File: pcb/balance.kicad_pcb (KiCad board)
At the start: 2 copper layers, 7 x 6 mm, 42 parts, among them J1 Resistive_Touch, J2 JTAG, J3 Conn_01x04_Male, J4 PJ-102AH, J5 UART (Bluetooth), J6 Conn_02x03_Top_Bottom, J7 Conn_02x05_Top_Bottom, M1 Motor_Servo, M2 Motor_Servo, Q1 MMBT3904, Q2 MMBT3904, Q3 MMBT3904, SW1 SW_Push, U1 TM4C123GH6PMI, U2 LM2937xS, Y1 16MHz

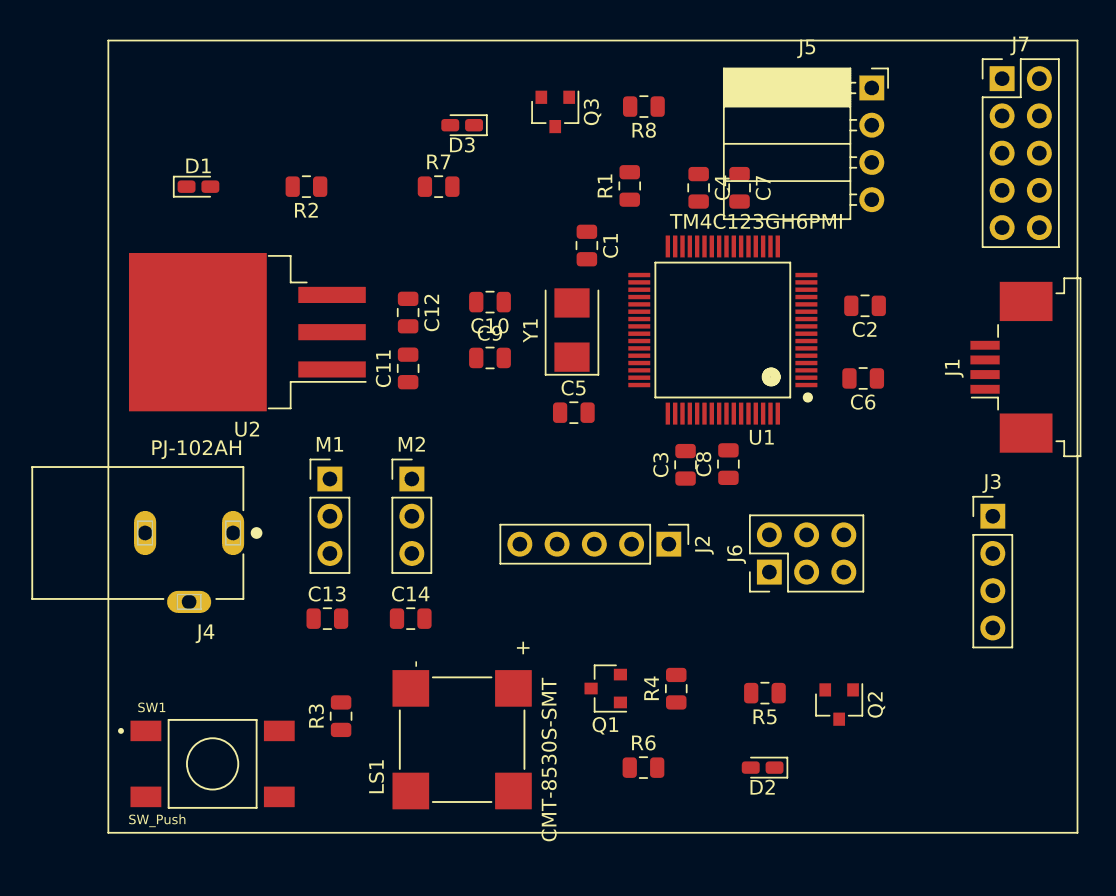
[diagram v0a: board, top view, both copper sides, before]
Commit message: Route the board
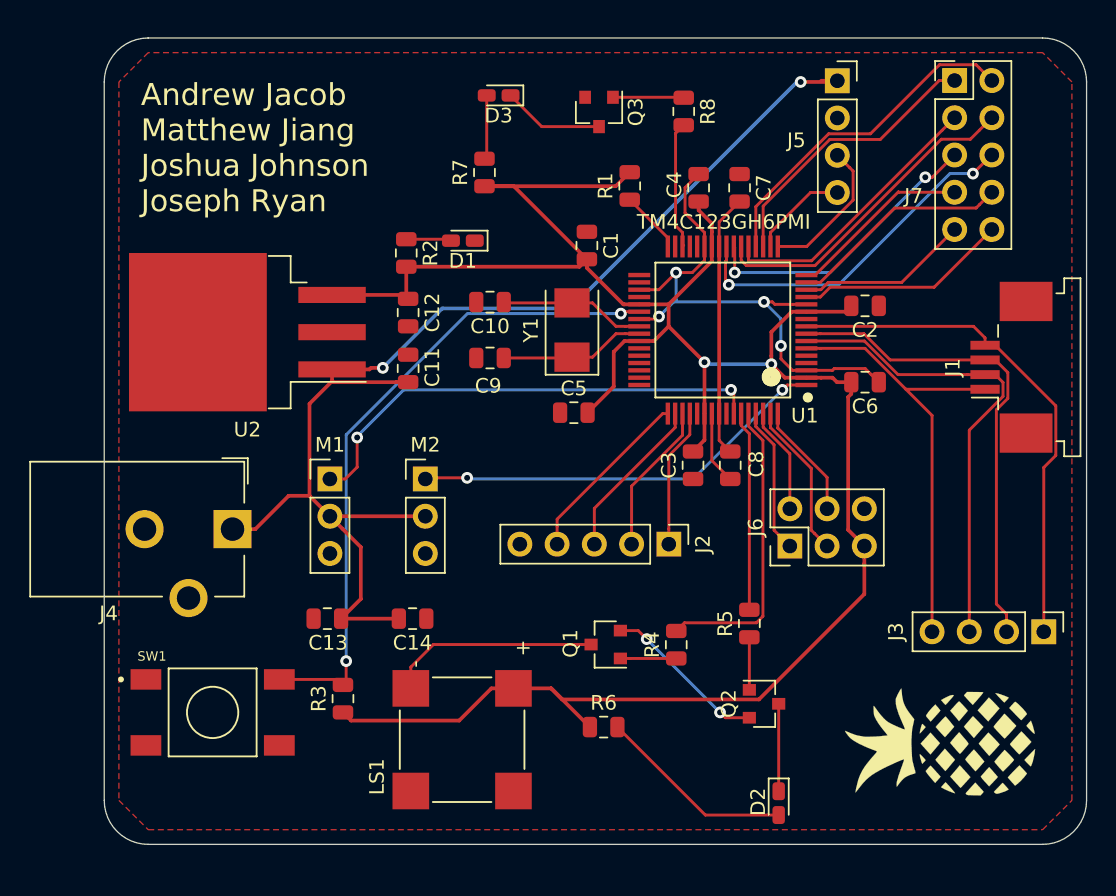
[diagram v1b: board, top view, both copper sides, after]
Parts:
- added G***: LOGO, pineapple:pineapple, F.Cu at (138.0, 150.0)
- J4: value PJ-102AH -> Barrel_Jack_Switch; footprint PJ-102AH:CUI_PJ-102AH -> Connector_BarrelJack:BarrelJack_CUI_PJ-102AH_Horizontal
- J5: footprint Connector_PinSocket_2.54mm:PinSocket_1x04_P2.54mm_Horizontal -> Connector_PinSocket_2.54mm:PinSocket_1x04_P2.54mm_Vertical
- moved D1 18.4 mm to (105.5, 115.8), turned to 180 degrees
- moved J3 8.61 mm to (145.1, 142.5), turned to 270 degrees
- moved R2 8.18 mm to (101.6, 116.7), turned to 90 degrees
- moved J4 6.47 mm to (89.8, 135.5), turned to 270 degrees
- moved Q2 5.13 mm to (126.0, 147.4), turned to 0 degrees
- moved R5 4.86 mm to (125.0, 141.9), turned to 90 degrees
- moved R6 3.88 mm to (115.1, 149.0)
- moved SW1 3.51 mm to (88.4, 148.0)
- moved R7 3.27 mm to (106.9, 111.2), turned to 90 degrees
- moved J7 3.24 mm to (139.0, 104.9)
- moved D3 3.21 mm to (107.9, 105.9)
- moved Q1 3.00 mm to (115.2, 143.4)
- moved R4 3.00 mm to (120.0, 143.4)
- moved Q3 2.99 mm to (114.7, 107.0)
- moved R8 2.74 mm to (120.5, 107.0), turned to 90 degrees
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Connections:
- J7 pad 8: /PC6 -> /PC5
- U1 pad 15: (no net) -> /PC5
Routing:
- net +3V3: track 0.00 -> 153.6 mm, vias 0 -> 2
- net +5V: track 0.00 -> 87.0 mm, vias 0 -> 2
- net GND: track 0.00 -> 54.2 mm, vias 0 -> 6
- net /RESET: track 0.00 -> 45.1 mm, vias 0 -> 2
- net Net-(J1-Pad4): track 0.00 -> 35.3 mm
- net Net-(J1-Pad3): track 0.00 -> 33.1 mm
- net /Servo0: track 0.00 -> 32.8 mm, vias 0 -> 2
- net Net-(J1-Pad2): track 0.00 -> 32.5 mm
- net Net-(J1-Pad1): track 0.00 -> 30.6 mm
- net /Servo1: track 0.00 -> 28.7 mm, vias 0 -> 2
- net /PA7: track 0.00 -> 24.4 mm, vias 0 -> 2
- net /PA3: track 0.00 -> 23.3 mm
- net /PA5: track 0.00 -> 22.4 mm
- net /BZZZ: track 0.00 -> 20.6 mm
- net /PA6: track 0.00 -> 20.1 mm, vias 0 -> 2
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- added copper zone on F.Cu, net GND
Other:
- board size 7 x 6 mm -> 67 x 55 mm
- net class Default: clearance 0.2 -> 0.127; trace_width 0.25 -> 0.2
- net class Power added: clearance 0.127, trace_width 0.254, via_dia 0.8, via_drill 0.4
- rule trace_clearance: 0.2 -> 0.127
- board text added: "Andrew Jacob Matthew Jiang Joshua Johnson Joseph Ryan"
